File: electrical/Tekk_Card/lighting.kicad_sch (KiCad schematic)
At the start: 16 parts

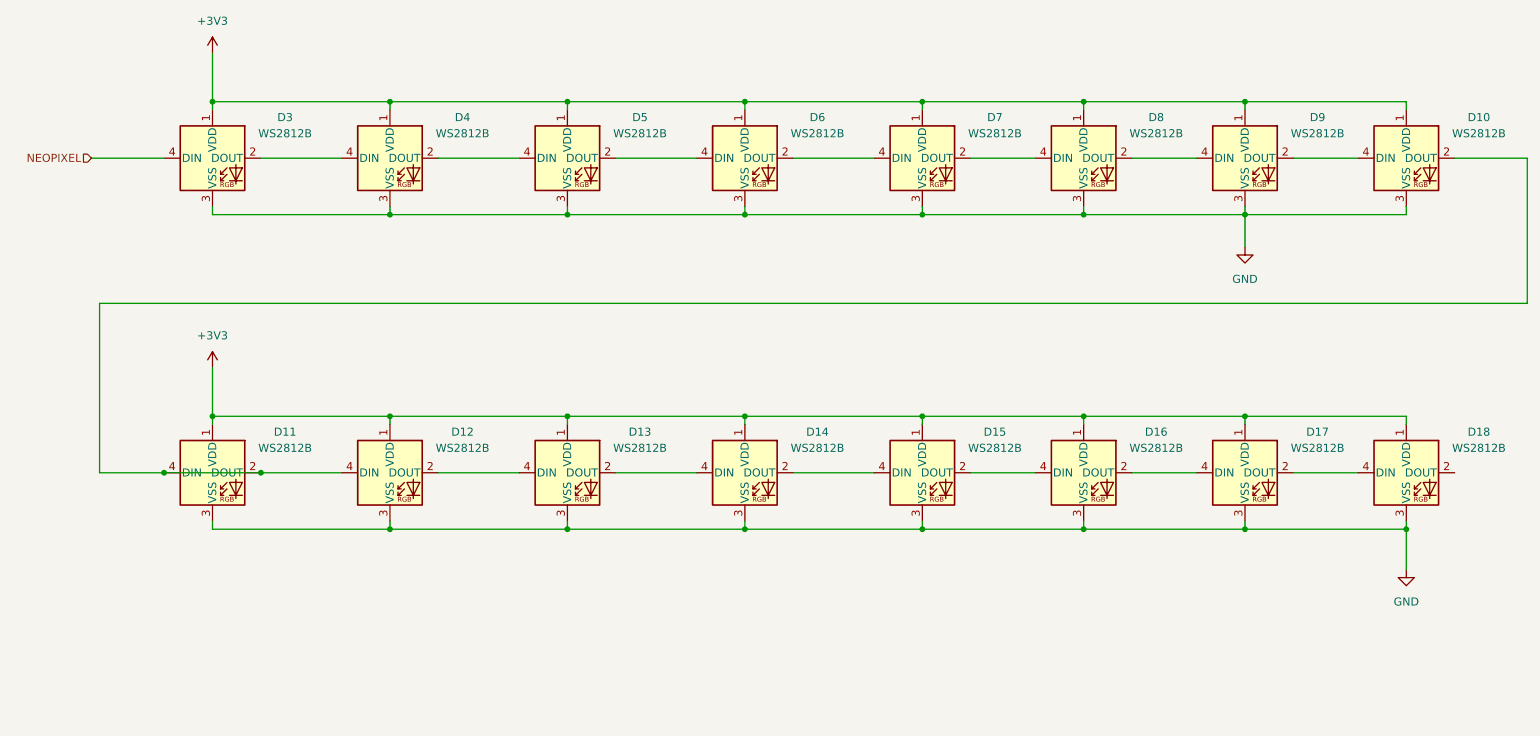
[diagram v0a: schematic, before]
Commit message: Continue initial prototype
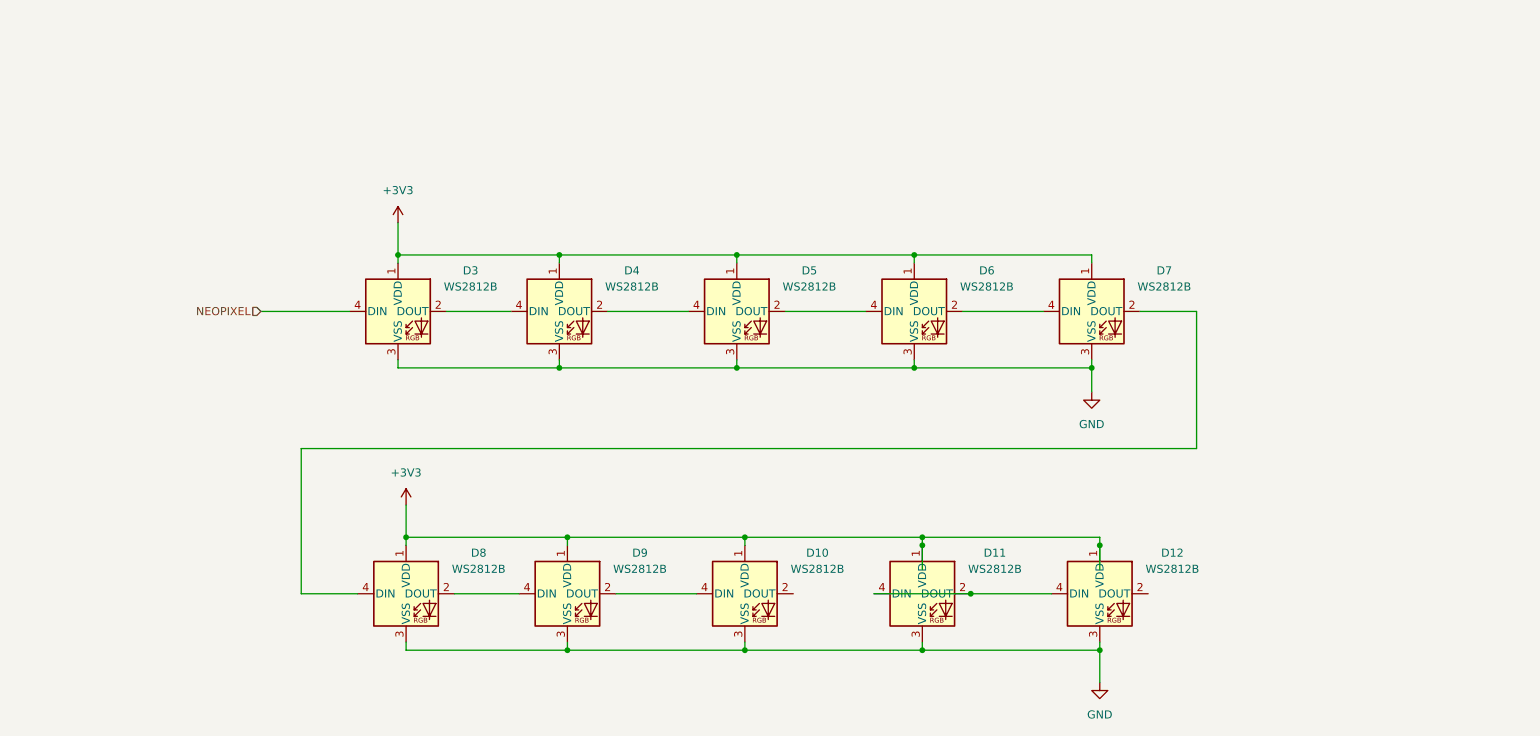
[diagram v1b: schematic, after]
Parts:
- removed D13, D14, D15, D16, D17, D18: WS2812B, LED_SMD:LED_WS2812B_PLCC4_5.0x5.0mm_P3.2mm, symbol LED:WS2812B
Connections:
- net at D11.2 (DOUT), D11.4 (DIN), D12.4 (DIN): no longer D10.2 (DOUT)
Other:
- moved on the sheet: D10, D11, D12, D3, D4, D5, D6, D7, D8, D9
